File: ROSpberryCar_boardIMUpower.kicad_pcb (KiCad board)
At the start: 2 copper layers, 32.3 x 33.3 mm, 14 parts, among them P1 CONN_5, P2 CONN_6, P3 RASPI_CONN, P4 CONN_2, P5 CONN_5

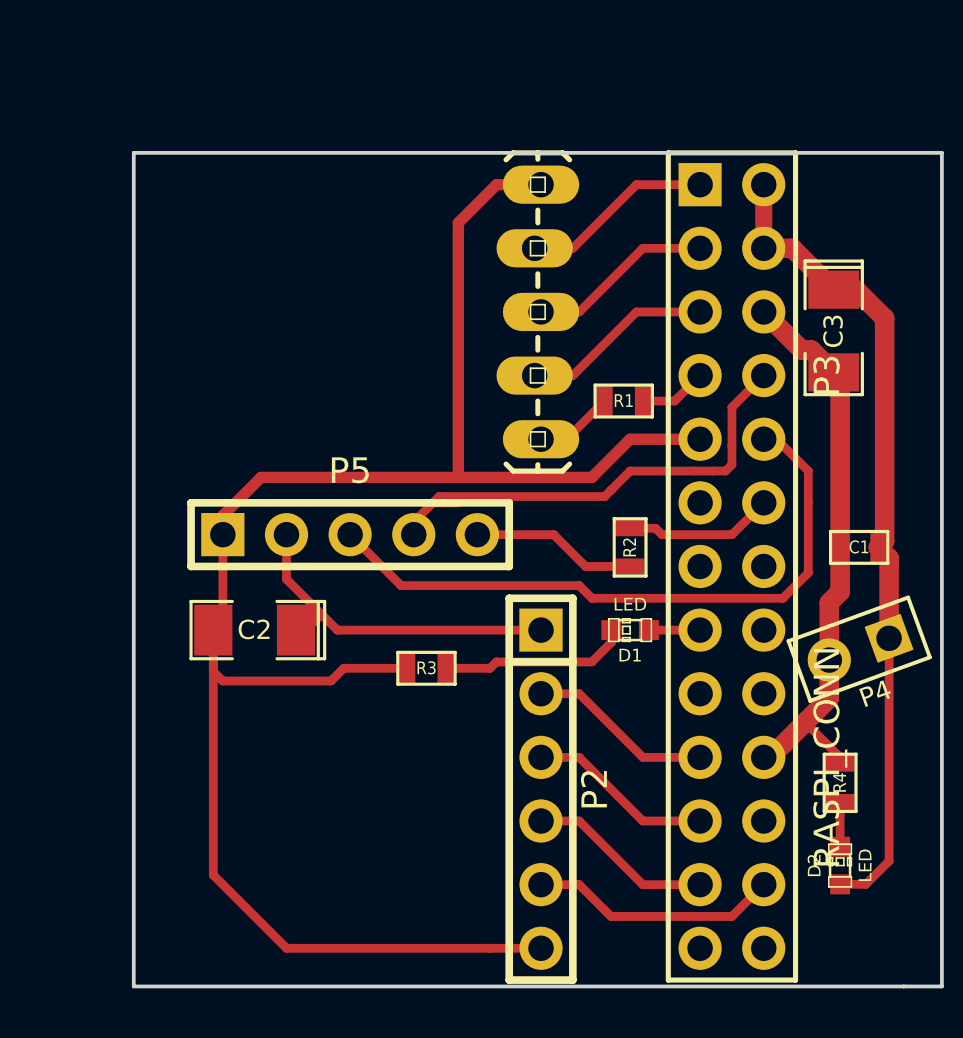
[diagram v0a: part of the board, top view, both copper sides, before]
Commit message: v2
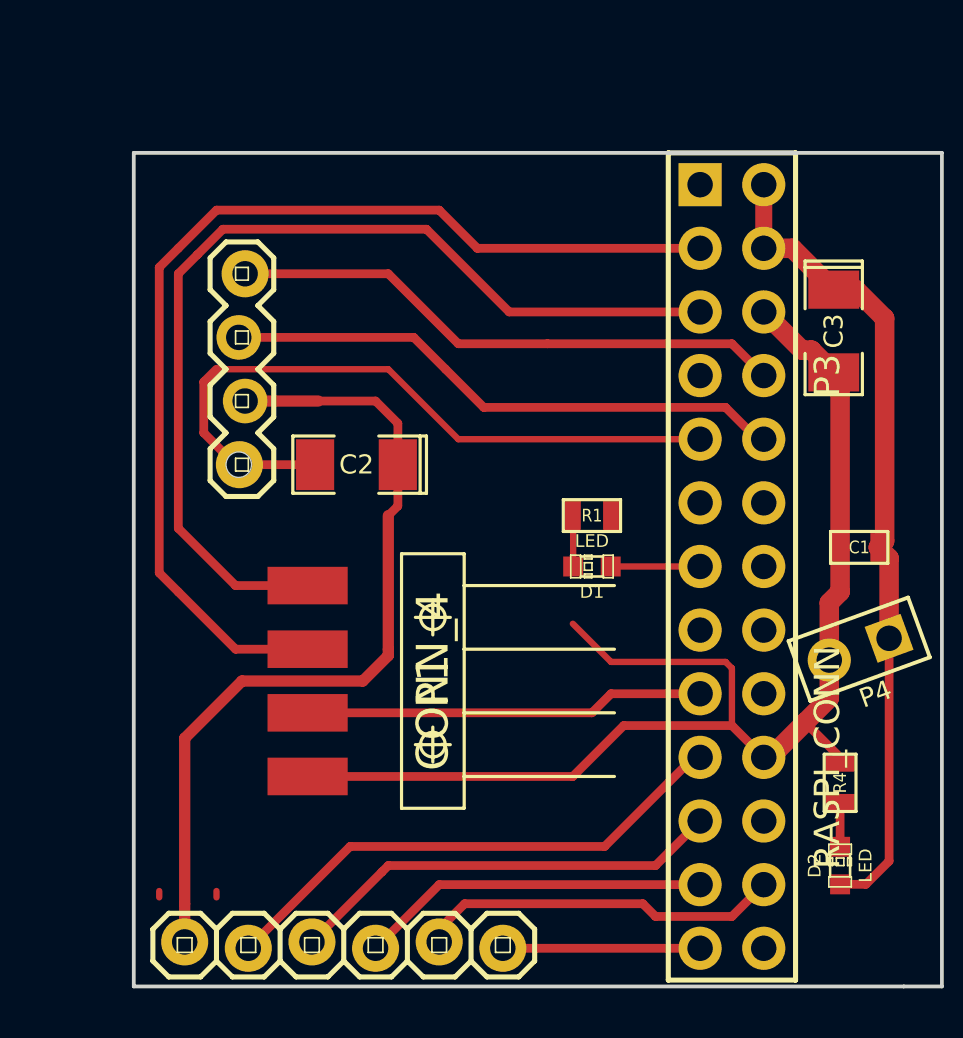
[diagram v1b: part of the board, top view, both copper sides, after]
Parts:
- removed R2, R3: R, SM0603
- P1: value CONN_5 -> CONN_4; footprint SparkFun-1X05_LOCK_LONGPADS -> SparkFun-1X04-SMD
- P2: footprint PIN_ARRAY-6X1 -> SparkFun-1X06_LOCK
- P5: value CONN_5 -> CONN_4; footprint PIN_ARRAY_5x1 -> SparkFun-1X04_LOCK
- moved P1 20.3 mm to (178.6, 108.7), turned to 90 degrees
- moved P2 15.5 mm to (168.7, 119.1), turned to 0 degrees
- moved C2 7.75 mm to (175.5, 100.1)
- moved P5 5.14 mm to (170.9, 100.1), turned to 90 degrees
- moved R1 4.75 mm to (184.9, 102.1), turned to 180 degrees
- moved D1 2.96 mm to (184.9, 104.1)
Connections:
- C2 pad 2: N-0000022 (its old number) -> /gnd
- D1 pad 1: N-000006 (its old number) -> N-000003
- D1 pad 2: N-000005 (its old number) -> N-000002
- P1 pad 1: N-0000022 (its old number) -> /gnd
- P1 pad 2: N-0000027 -> /3v3_2
- P2 pad 6: N-0000022 (its old number) -> N-000004
- P3 pad 1: N-0000027 -> N-0000024
- P3 pad 13: N-0000017 (its old number) -> N-000003
- P3 pad 15: N-000006 (its old number) -> N-0000014
- P3 pad 17: N-0000011 (its old number) -> /3v3_2
- P3 pad 25: N-0000014 -> N-000004
- P3 pad 7: N-000003 -> N-0000021
- P3 pad 9: N-0000022 (its old number) -> /gnd
- P5 pad 1: N-0000022 (its old number) -> /gnd
- R1 pad 1: N-000002 -> /gnd
- R1 pad 2: N-000003 -> N-000002
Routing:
- net N-0000022 (its old number): track 73.0 -> 0.00 mm
- net /gnd: track 22.9 -> 80.3 mm
- net N-0000023: track 7.40 -> 42.5 mm
- net N-0000022: track 7.66 -> 39.2 mm
- net N-000006: track 14.1 -> 33.5 mm
- net /3v3_2: track 0.00 -> 16.0 mm
- net N-0000010: track 7.40 -> 21.2 mm
- net N-000009: track 7.40 -> 17.5 mm
- net N-000004: track 0.00 -> 7.87 mm
- net N-0000027: track 7.66 -> 0.00 mm
- net N-000005 (its old number): track 7.54 -> 0.00 mm
- net N-0000028: track 6.62 -> 0.00 mm
- net N-0000016: track 7.40 -> 14.0 mm
- net N-0000018: track 5.97 -> 0.00 mm
- net N-000001: track 9.94 -> 14.6 mm
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- added copper zone on F.Cu, net /gnd
- removed copper zone on F.Cu, net (none)
